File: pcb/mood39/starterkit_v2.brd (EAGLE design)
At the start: 32 x 32 mm, 19 parts, among them IC1 TINY85, IC2 LP2950

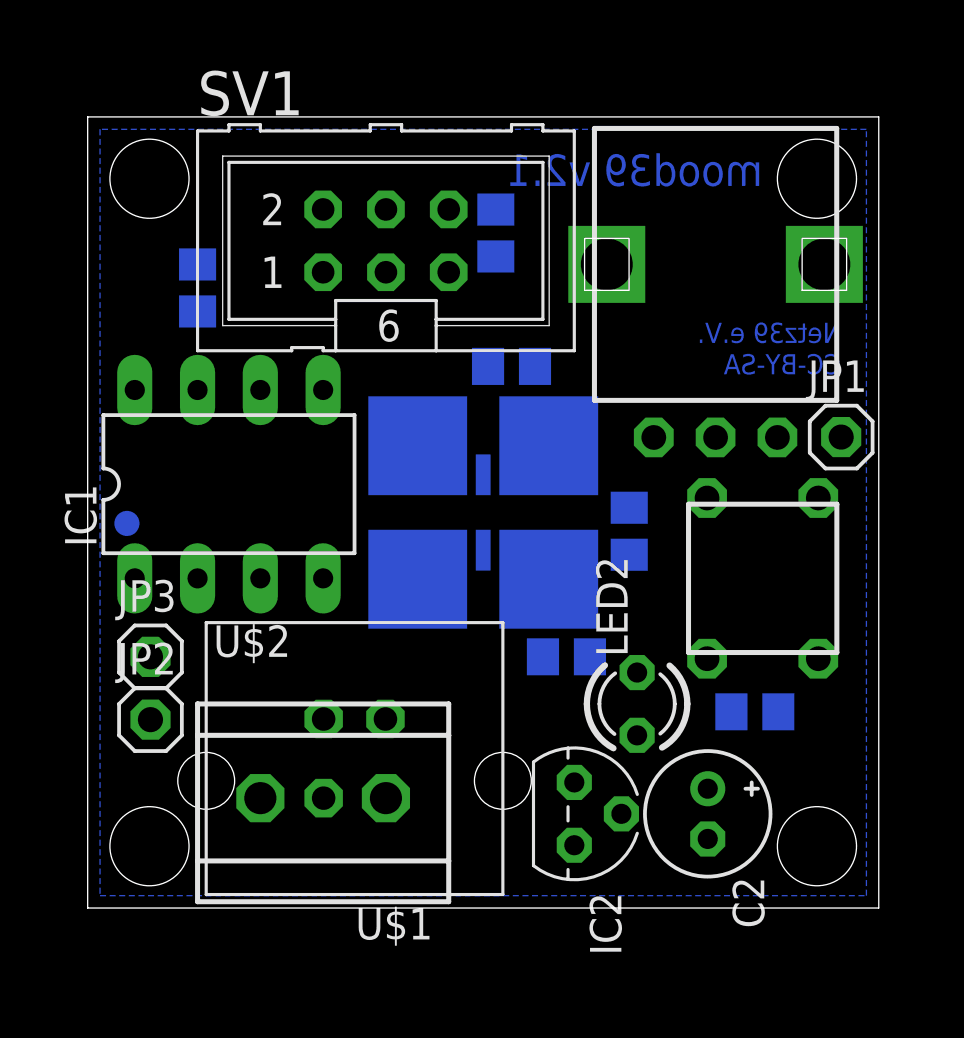
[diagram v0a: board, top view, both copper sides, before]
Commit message: try another puzzle
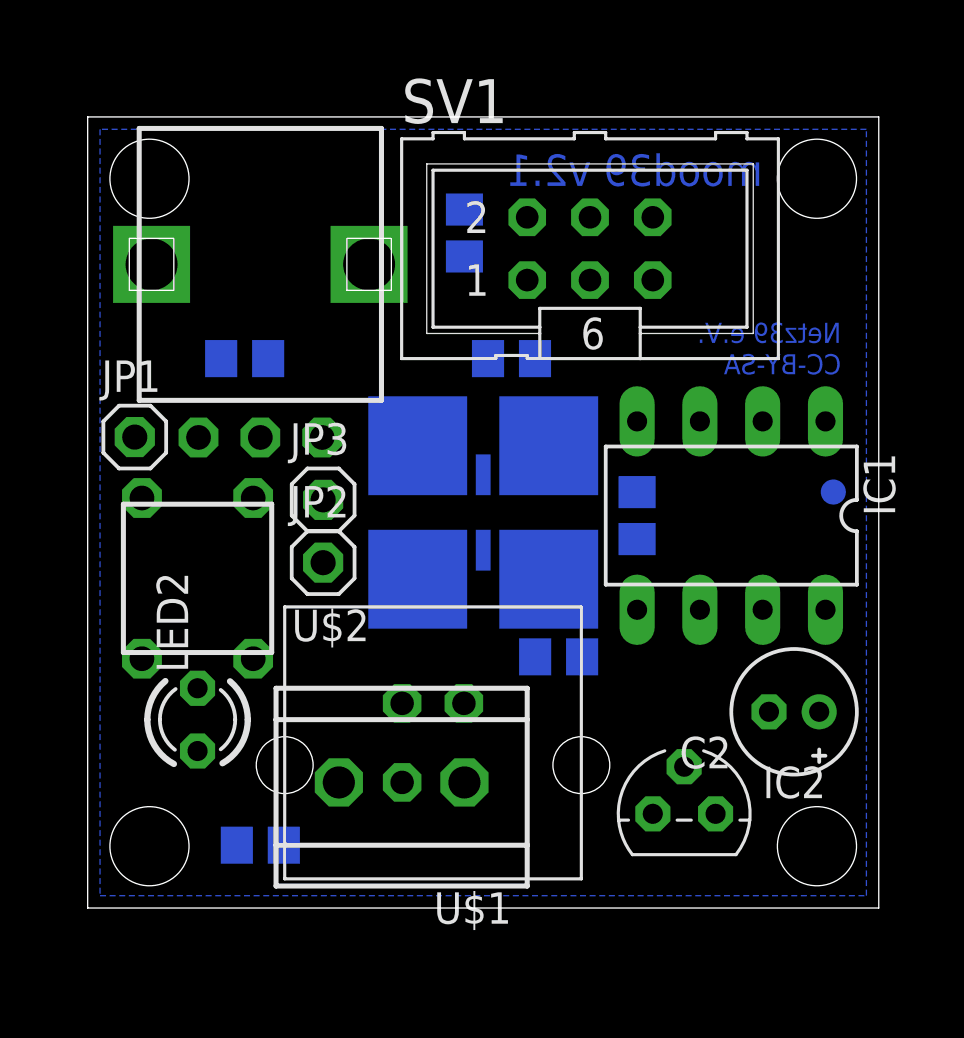
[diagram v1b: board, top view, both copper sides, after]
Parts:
- moved JP1 28.6 mm to (1.91, 19.1)
- moved S1 22.9 mm to (4.45, 13.3)
- moved R6 20.7 mm to (6.99, 2.54)
- moved IC1 20.4 mm to (26.0, 15.9), turned to 180 degrees
- moved R5 18.4 mm to (6.99, 26.0)
- moved LED2 17.8 mm to (4.45, 7.62)
- moved JP2 9.44 mm to (9.53, 14.0)
- moved JP3 9.44 mm to (9.53, 16.5)
- moved SV1 8.26 mm to (20.3, 26.7)
- moved C2 5.41 mm to (28.6, 7.94), turned to 180 degrees
- moved IC2 4.45 mm to (24.1, 3.81), turned to 0 degrees
- moved C1 3.43 mm to (6.35, 22.2), turned to 0 degrees
- moved U$2 3.24 mm to (14.0, 5.08)
- moved U$1 3.24 mm to (12.7, 5.08)
- moved R1 1.27 mm to (15.2, 27.3), turned to 270 degrees
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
